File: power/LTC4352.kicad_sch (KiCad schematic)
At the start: 15 parts, among them Q1 Si7336ADP, U1 LTC4352CMS

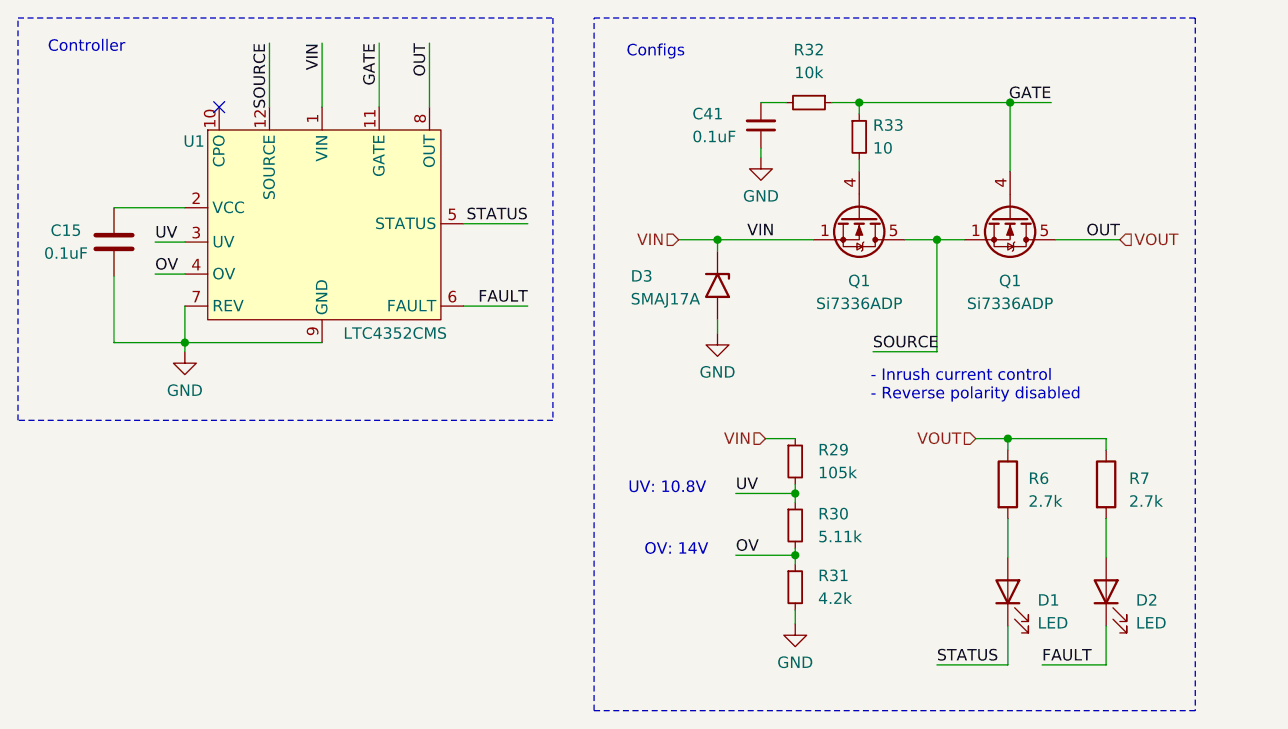
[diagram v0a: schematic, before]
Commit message: Feat[power]: v2.1 schematic complete
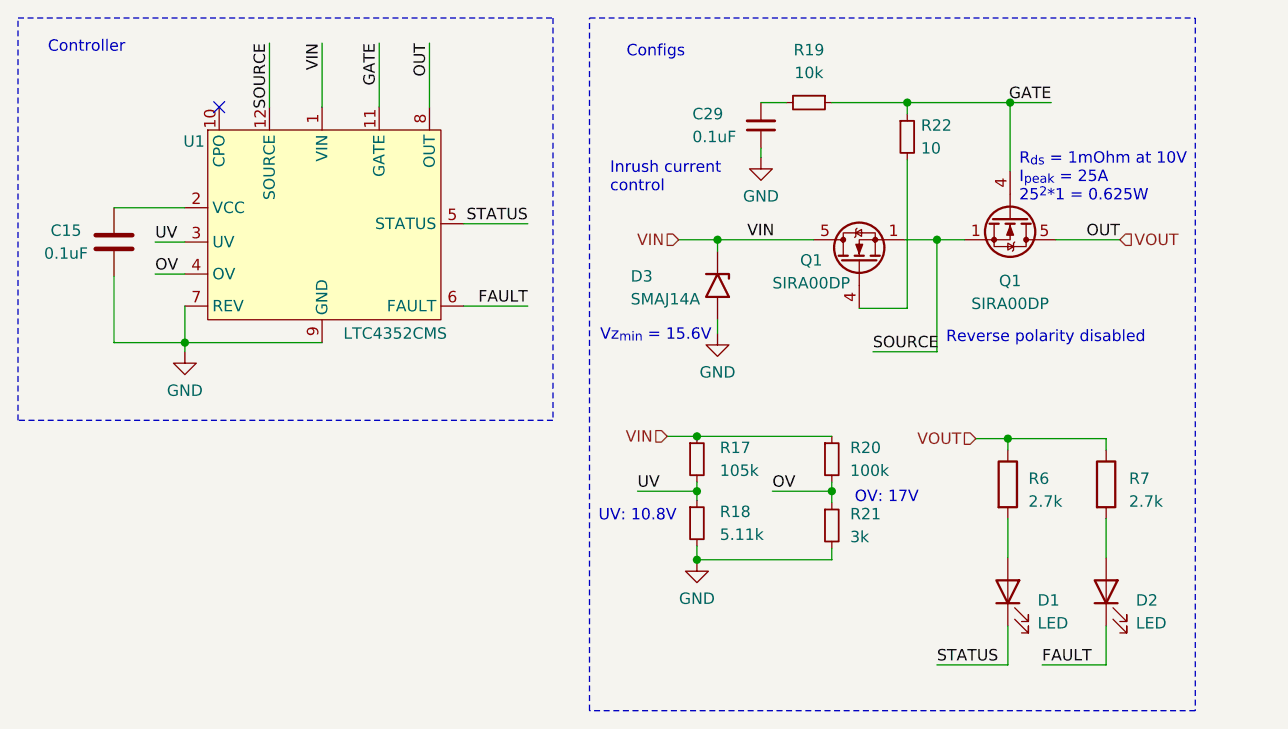
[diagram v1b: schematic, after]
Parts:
- removed R31: 4.2k, Resistor_SMD:R_0603_1608Metric, symbol Device:R_Small
- added R20: 100k, Resistor_SMD:R_0603_1608Metric, symbol Device:R_Small
- added R21: 3k, Resistor_SMD:R_0603_1608Metric, symbol Device:R_Small
- D3: value SMAJ17A -> SMAJ14A
- Q1: value Si7336ADP -> SIRA00DP
- renumbered C41 to C29, R29 to R17, R30 to R18, R32 to R19, R33 to R22
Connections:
- net GND: now also R18.2, R21.2
- net OV: now also R20.2, R21.1; no longer R18.2
- net SOURCE: now also Q1.1 (S), Q1.2 (S), Q1.3 (S); no longer Q1.5 (D)
- net VIN: now also Q1.5 (D), R20.1; no longer Q1.1 (S), Q1.2 (S), Q1.3 (S)
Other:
- note added: "Inrush current control"
- note added: "OV: 17V"
- note added: "R_{ds} = 1mOhm at 10V I_{peak} = 25A 25^{2}*1 = 0.625W"
- note added: "Reverse polarity disabled"
- note added: "Vz_{min} = 15.6V"
- note removed: "- Inrush current control - Reverse polarity disabled"
- note removed: "OV: 14V"
- moved on the sheet: Q1, R17, R18, R22
